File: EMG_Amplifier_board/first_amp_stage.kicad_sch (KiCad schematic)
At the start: 12 parts, among them U2 INA333xxDGK, U3 LPV821DBVR

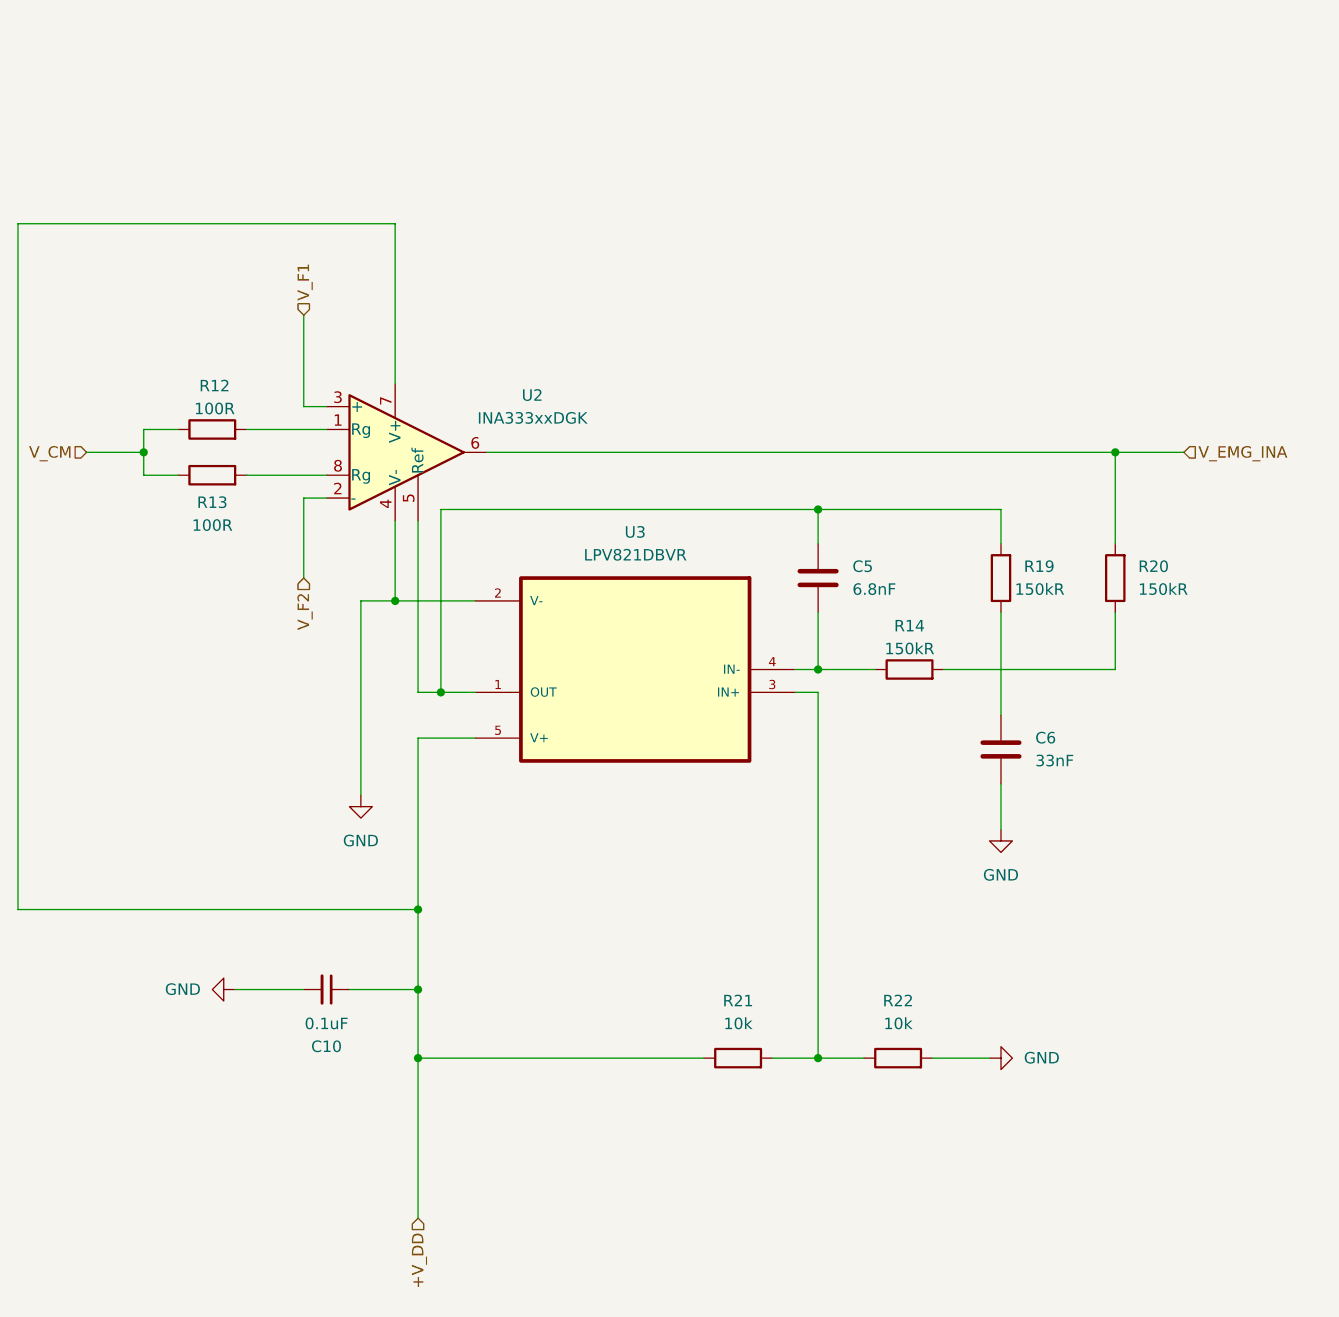
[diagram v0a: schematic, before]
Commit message: before working on one-sided design
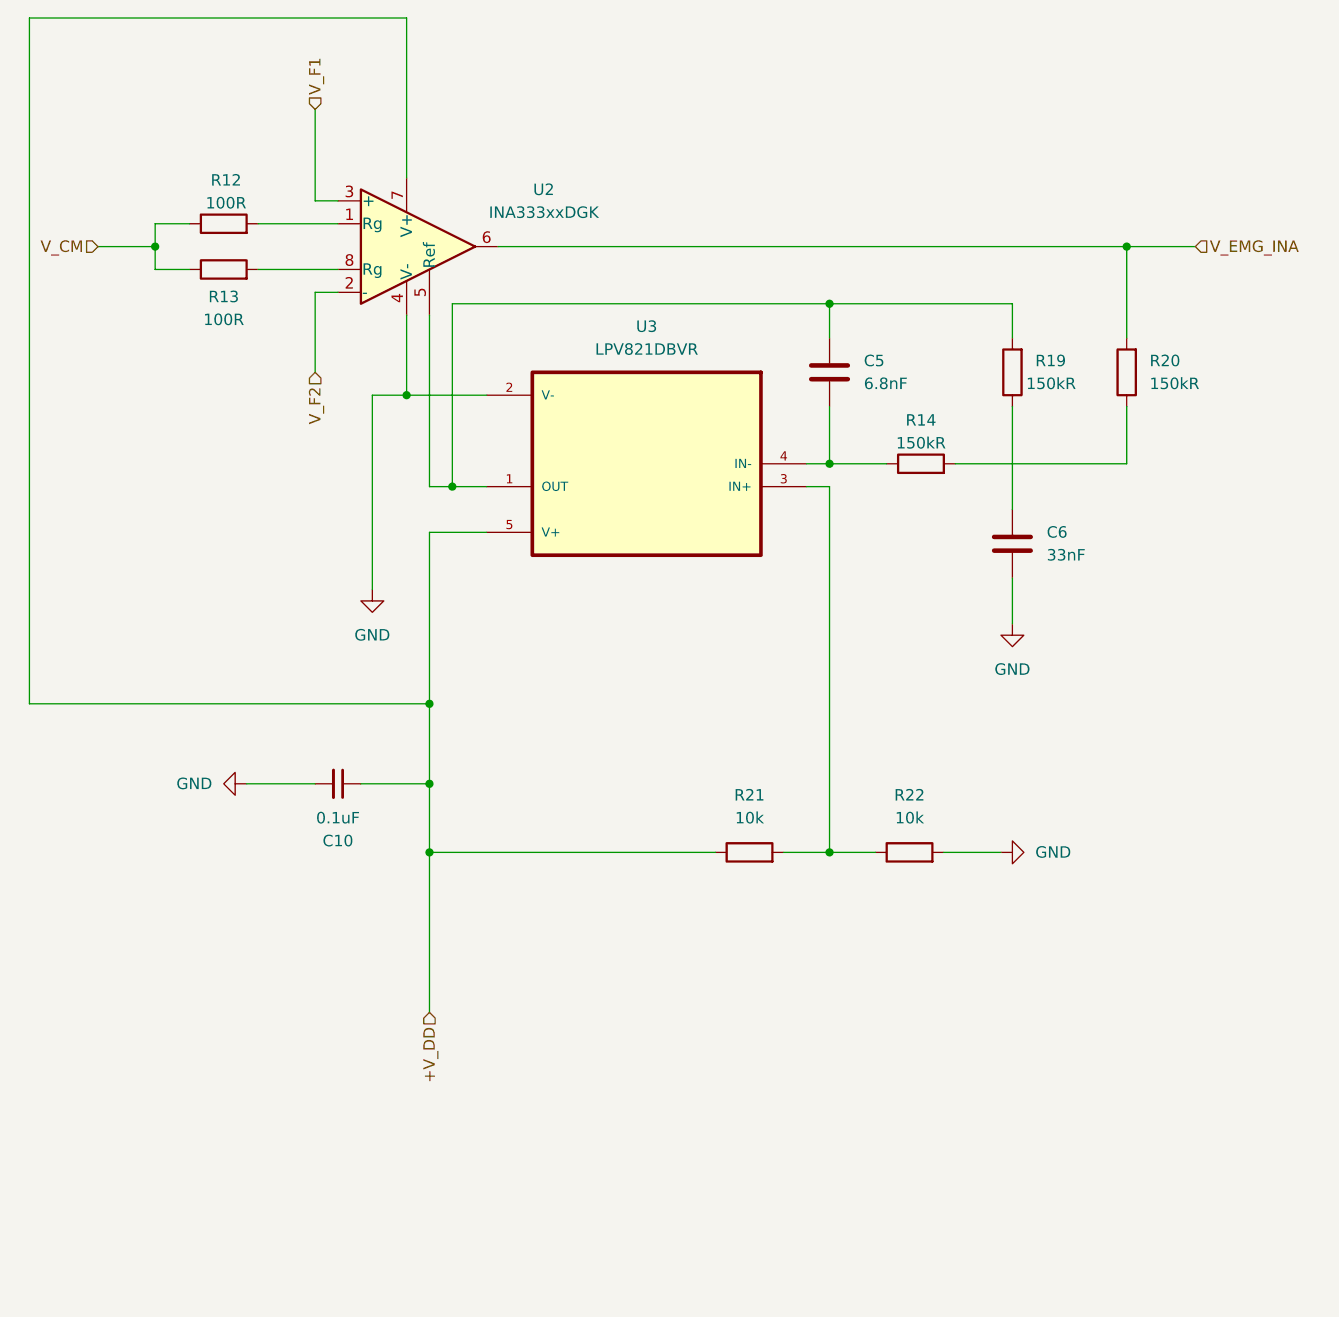
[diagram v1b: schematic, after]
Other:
- moved on the sheet: C10, C5, C6, R12, R13, R14, R19, R20, R21, R22, U2, U3
